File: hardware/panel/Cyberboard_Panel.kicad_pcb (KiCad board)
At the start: 4 copper layers, 51 x 44 mm, 136 parts, among them J1 Conn_01x20, J2 Conn_01x20, SW1 SW_Push, SW2 SW_Push, U1 SZYY0402Y_C434450, U10 XL-1005UBC_C22355736, U2 TPD2EUSB30, U3 NX2012SA-32.768KHZ-STD-MUB-2, U4 STM32WB55RGVx, U5 BQ24072RGT, U6 TPS631000DRLR, U7 ICM-42688-PC, U8 BMP580, U9 DFE252012P-1R0M=P2, X1 NX2016SA-32MHZ-STD-CZS-5

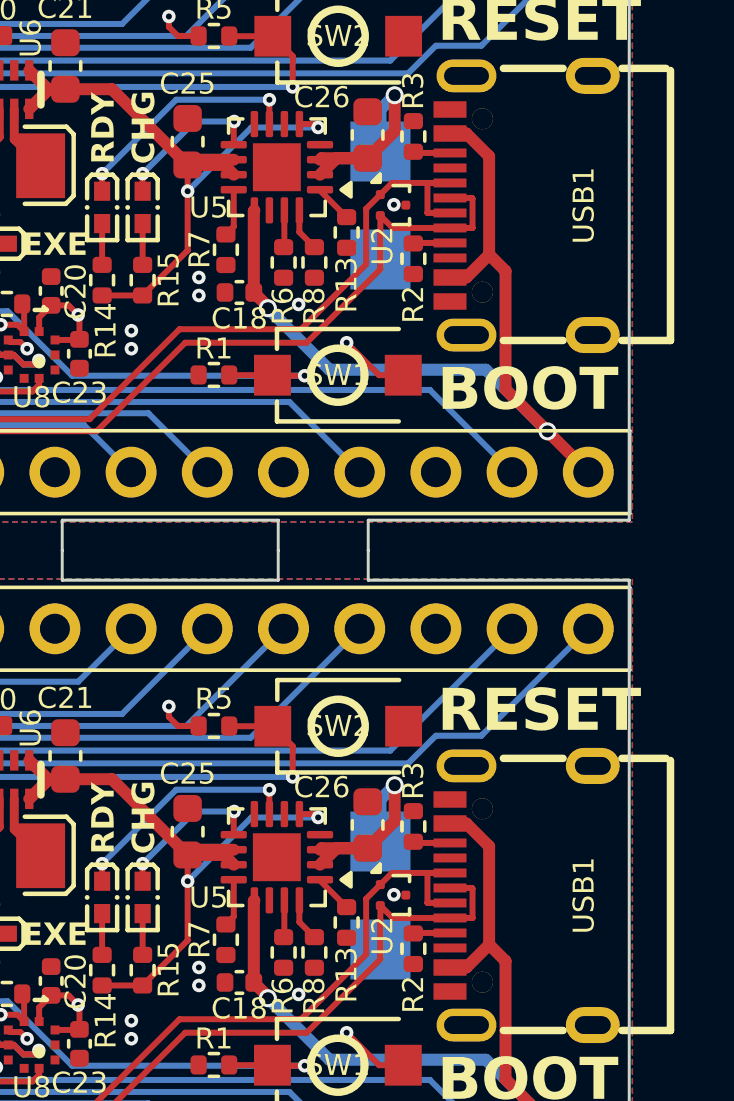
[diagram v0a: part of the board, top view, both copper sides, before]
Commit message: rounded corners and new renders and flyer
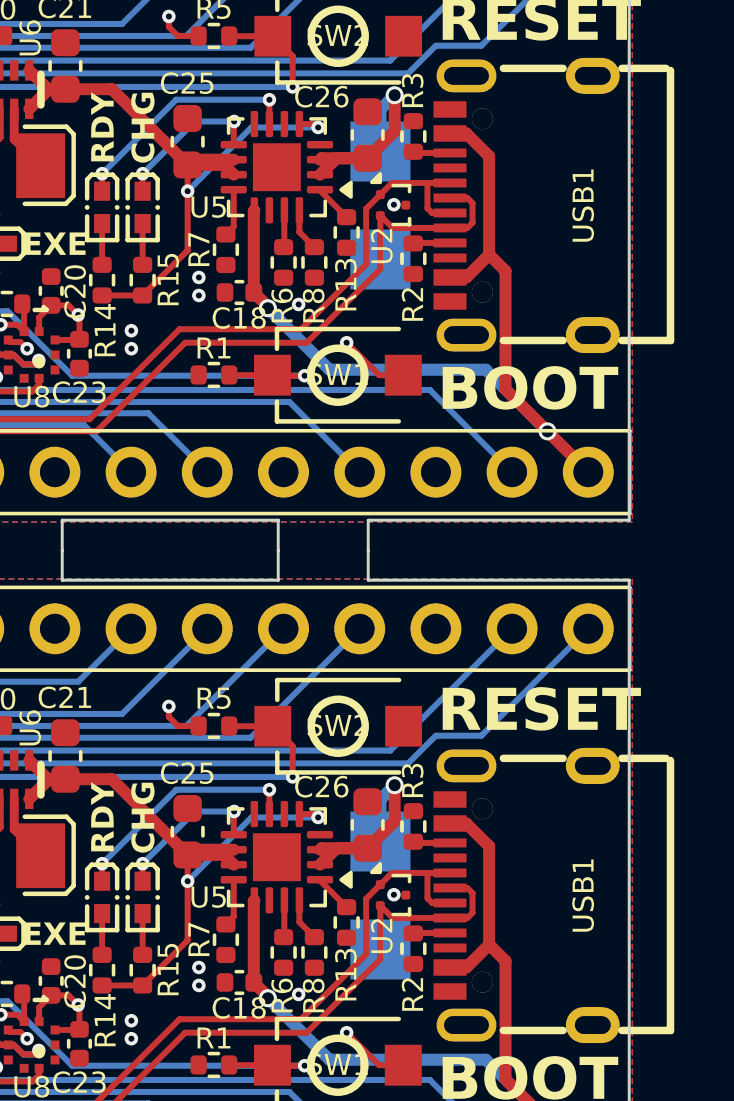
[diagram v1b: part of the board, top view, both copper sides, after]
